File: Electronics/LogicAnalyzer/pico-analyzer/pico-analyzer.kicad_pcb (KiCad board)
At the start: 4 copper layers, 78.7 x 76.2 mm, 69 parts, among them J1 Channels 0-5, J2 Channels 6-11, J3 Channels 12-17, J4 Channels 18-23, J5 USB_C_Receptacle_USB2.0_16P, SW1 SW_DP3T, U1 TXU0104PW, U2 TXU0104PW, U3 TXU0104PW, U4 TXU0104PW, U5 TXU0104PW, U6 TXU0104PW, U7 RP2040_Stamp

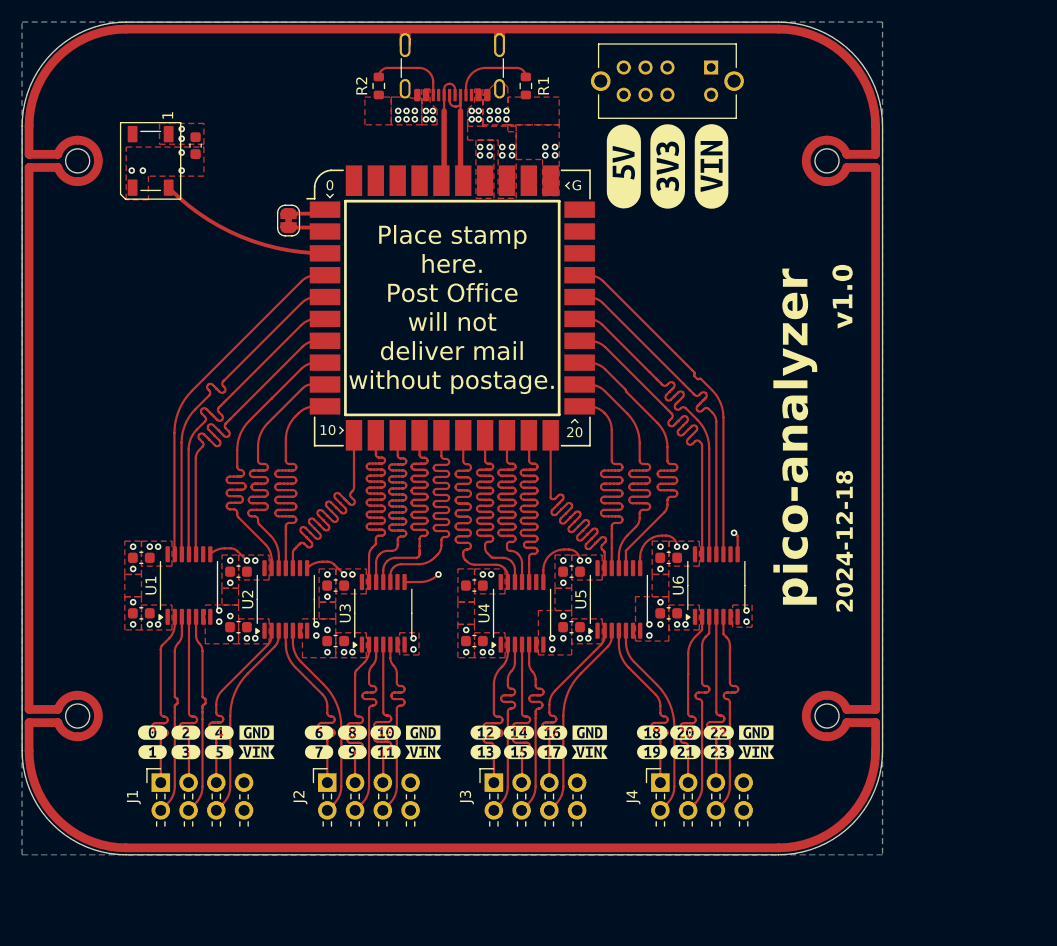
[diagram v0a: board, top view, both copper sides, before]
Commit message: Working on pico-analyzer v2
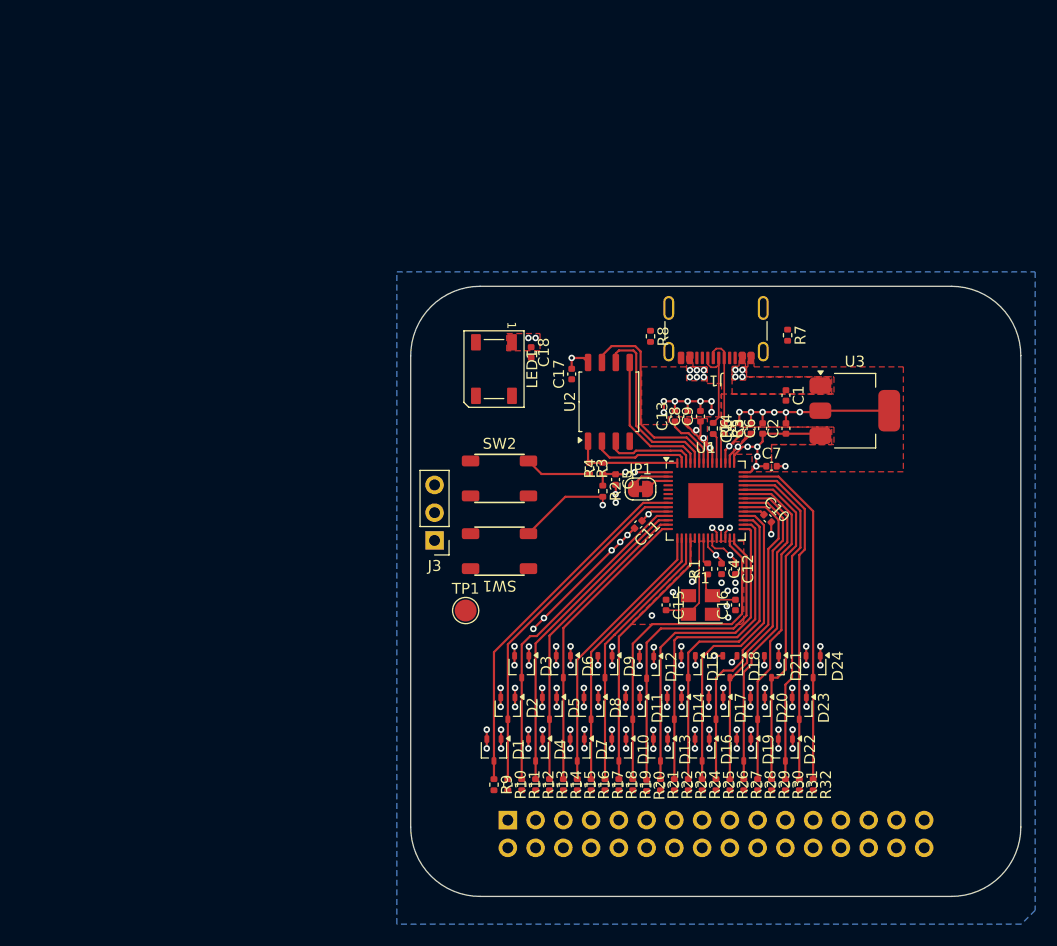
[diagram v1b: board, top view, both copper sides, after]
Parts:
- removed J4: Channels 18-23, pico-analyzer:PinHeader_2x04_P2.54mm_Horizontal
- removed J5: USB_C_Receptacle_USB2.0_16P, pico-analyzer:USB_C_Receptacle_GCT_USB4215-xx-A_16P
- removed MH (x4): MountingHole_2.2mm_M2_DIN965, MountingHole:MountingHole_2.2mm_M2_DIN965
- removed U4, U5, U6: TXU0104PW, Package_SO:TSSOP-14_4.4x5mm_P0.65mm
- removed U7: RP2040_Stamp, pico-analyzer:RP2xxx_Stamp_SMD
- removed kibuzzard-67631203: G***, kibuzzard-67631203
- removed kibuzzard-6763120A: G***, kibuzzard-6763120A
- removed kibuzzard-67631217: G***, kibuzzard-67631217
- removed kibuzzard-67631277: G***, kibuzzard-67631277
- removed kibuzzard-6763127F: G***, kibuzzard-6763127F
- removed kibuzzard-67631289: G***, kibuzzard-67631289
- removed kibuzzard-6763155B: G***, kibuzzard-6763155B
- removed kibuzzard-67631565: G***, kibuzzard-67631565
- removed kibuzzard-6763156D: G***, kibuzzard-6763156D
- removed kibuzzard-67631578: G***, kibuzzard-67631578
- removed kibuzzard-67631580: G***, kibuzzard-67631580
- removed kibuzzard-67631586: G***, kibuzzard-67631586
- removed kibuzzard-676315DE (x4): G***, kibuzzard-676315DE
- removed kibuzzard-67631617 (x4): G***, kibuzzard-67631617
- removed kibuzzard-67631703: G***, kibuzzard-67631703
- removed kibuzzard-6763170A: G***, kibuzzard-6763170A
- removed kibuzzard-67631748: G***, kibuzzard-67631748
- removed kibuzzard-6763175E: G***, kibuzzard-6763175E
- removed kibuzzard-67631765: G***, kibuzzard-67631765
- removed kibuzzard-67631771: G***, kibuzzard-67631771
- removed kibuzzard-676317E0: G***, kibuzzard-676317E0
- removed kibuzzard-676317E5: G***, kibuzzard-676317E5
- removed kibuzzard-676317E9: G***, kibuzzard-676317E9
- removed kibuzzard-676317ED: G***, kibuzzard-676317ED
- removed kibuzzard-676317F6: G***, kibuzzard-676317F6
- removed kibuzzard-67631801: G***, kibuzzard-67631801
- removed kibuzzard-67632017: G***, kibuzzard-67632017
- removed kibuzzard-6763201C: G***, kibuzzard-6763201C
- removed kibuzzard-67632021: G***, kibuzzard-67632021
- added C14: 0.1µF, Capacitor_SMD:C_0402_1005Metric, F.Cu at (141.8, 88.0)
- added C15: 15pF, Capacitor_SMD:C_0402_1005Metric, F.Cu at (135.1, 104.1)
- added C16: 15pF, Capacitor_SMD:C_0402_1005Metric, F.Cu at (141.5, 104.1)
- added C17: 0.1µF, Capacitor_SMD:C_0402_1005Metric, F.Cu at (126.5, 83.0)
- added C18: 0.1µF, Capacitor_SMD:C_0402_1005Metric, F.Cu at (122.8, 81.0)
- added D10: BAV99, Package_TO_SOT_SMD:SOT-323_SC-70, F.Cu at (130.8, 117.4)
- added D11: BAV99, Package_TO_SOT_SMD:SOT-323_SC-70, F.Cu at (132.1, 113.6)
- added D12: BAV99, Package_TO_SOT_SMD:SOT-323_SC-70, F.Cu at (133.3, 109.9)
- added D13: BAV99, Package_TO_SOT_SMD:SOT-323_SC-70, F.Cu at (134.6, 117.4)
- added D14: BAV99, Package_TO_SOT_SMD:SOT-323_SC-70, F.Cu at (135.9, 113.6)
- added D15: BAV99, Package_TO_SOT_SMD:SOT-323_SC-70, F.Cu at (137.2, 109.8)
- added D16: BAV99, Package_TO_SOT_SMD:SOT-323_SC-70, F.Cu at (138.4, 117.4)
- added D17: BAV99, Package_TO_SOT_SMD:SOT-323_SC-70, F.Cu at (139.7, 113.6)
- added D18: BAV99, Package_TO_SOT_SMD:SOT-323_SC-70, F.Cu at (141.0, 109.8)
- added D19: BAV99, Package_TO_SOT_SMD:SOT-323_SC-70, F.Cu at (142.2, 117.4)
- added D2: BAV99, Package_TO_SOT_SMD:SOT-323_SC-70, F.Cu at (120.7, 113.6)
- added D20: BAV99, Package_TO_SOT_SMD:SOT-323_SC-70, F.Cu at (143.5, 113.6)
- added D21: BAV99, Package_TO_SOT_SMD:SOT-323_SC-70, F.Cu at (144.8, 109.8)
- added D22: BAV99, Package_TO_SOT_SMD:SOT-323_SC-70, F.Cu at (146.1, 117.4)
- added D23: BAV99, Package_TO_SOT_SMD:SOT-323_SC-70, F.Cu at (147.3, 113.6)
- added D24: BAV99, Package_TO_SOT_SMD:SOT-323_SC-70, F.Cu at (148.6, 109.8)
- added D3: BAV99, Package_TO_SOT_SMD:SOT-323_SC-70, F.Cu at (121.9, 109.8)
- added D4: BAV99, Package_TO_SOT_SMD:SOT-323_SC-70, F.Cu at (123.2, 117.4)
- added D5: BAV99, Package_TO_SOT_SMD:SOT-323_SC-70, F.Cu at (124.5, 113.6)
- added D6: BAV99, Package_TO_SOT_SMD:SOT-323_SC-70, F.Cu at (125.7, 109.8)
- added D7: BAV99, Package_TO_SOT_SMD:SOT-323_SC-70, F.Cu at (127.0, 117.4)
- added D8: BAV99, Package_TO_SOT_SMD:SOT-323_SC-70, F.Cu at (128.3, 113.6)
- added D9: BAV99, Package_TO_SOT_SMD:SOT-323_SC-70, F.Cu at (129.5, 109.8)
- added LED1: WS2812B, LED_SMD:LED_WS2812B_PLCC4_5.0x5.0mm_P3.2mm, F.Cu at (119.4, 82.5)
- added R10: 220, Resistor_SMD:R_0402_1005Metric, F.Cu at (120.7, 120.6)
- added R11: 220, Resistor_SMD:R_0402_1005Metric, F.Cu at (121.9, 120.6)
- added R12: 220, Resistor_SMD:R_0402_1005Metric, F.Cu at (123.2, 120.6)
- added R13: 220, Resistor_SMD:R_0402_1005Metric, F.Cu at (124.5, 120.6)
- added R14: 220, Resistor_SMD:R_0402_1005Metric, F.Cu at (125.7, 120.6)
- added R15: 220, Resistor_SMD:R_0402_1005Metric, F.Cu at (127.0, 120.6)
- added R16: 220, Resistor_SMD:R_0402_1005Metric, F.Cu at (128.3, 120.6)
- added R17: 220, Resistor_SMD:R_0402_1005Metric, F.Cu at (129.5, 120.6)
- added R18: 220, Resistor_SMD:R_0402_1005Metric, F.Cu at (130.8, 120.6)
- added R19: 220, Resistor_SMD:R_0402_1005Metric, F.Cu at (132.1, 120.6)
- added R20: 220, Resistor_SMD:R_0402_1005Metric, F.Cu at (133.3, 120.7)
- added R21: 220, Resistor_SMD:R_0402_1005Metric, F.Cu at (134.6, 120.6)
- added R22: 220, Resistor_SMD:R_0402_1005Metric, F.Cu at (135.9, 120.6)
- added R23: 220, Resistor_SMD:R_0402_1005Metric, F.Cu at (137.2, 120.6)
- added R24: 220, Resistor_SMD:R_0402_1005Metric, F.Cu at (138.4, 120.6)
- added R25: 220, Resistor_SMD:R_0402_1005Metric, F.Cu at (139.7, 120.6)
- added R26: 220, Resistor_SMD:R_0402_1005Metric, F.Cu at (141.0, 120.6)
- added R27: 220, Resistor_SMD:R_0402_1005Metric, F.Cu at (142.2, 120.6)
- added R28: 220, Resistor_SMD:R_0402_1005Metric, F.Cu at (143.5, 120.6)
- added R29: 220, Resistor_SMD:R_0402_1005Metric, F.Cu at (144.8, 120.6)
- added R3: 1K, Resistor_SMD:R_0402_1005Metric, F.Cu at (128.1, 91.6)
- added R30: 220, Resistor_SMD:R_0402_1005Metric, F.Cu at (146.1, 120.6)
- added R31: 220, Resistor_SMD:R_0402_1005Metric, F.Cu at (147.3, 120.6)
- added R32: 220, Resistor_SMD:R_0402_1005Metric, F.Cu at (148.6, 120.6)
- added R4: 10K, Resistor_SMD:R_0402_1005Metric, F.Cu at (129.3, 91.6)
- added R5: 27R, Resistor_SMD:R_0402_1005Metric, F.Cu at (140.5, 88.0)
- added R6: 27R, Resistor_SMD:R_0402_1005Metric, F.Cu at (139.4, 88.0)
- added R7: 5K1, Resistor_SMD:R_0402_1005Metric, F.Cu at (146.3, 79.5)
- added R8: 5K1, Resistor_SMD:R_0402_1005Metric, F.Cu at (133.7, 79.6)
- added R9: 220, Resistor_SMD:R_0402_1005Metric, F.Cu at (119.4, 120.6)
- added SW2: BOOT, UPL-Switches:Button_Push_SPST_C&K_PTS647Sx38SMTR2LFS, F.Cu at (119.9, 92.6)
- added TP1: TESTEN, TestPoint:TestPoint_Pad_D2.0mm, F.Cu at (116.8, 104.6)
- added Y1: ABM8-272-T3, Crystal:Crystal_SMD_Abracon_ABM8G-4Pin_3.2x2.5mm, F.Cu at (138.3, 104.1)
- C1: value 100nF -> 4.7µF; footprint Capacitor_SMD:C_0603_1608Metric -> Capacitor_SMD:C_0402_1005Metric
- C10, C11, C13, C4, C5, C6, C7, C8, C9: value C_Small -> 0.1µF; footprint Capacitor_SMD:C_0603_1608Metric -> Capacitor_SMD:C_0402_1005Metric
- C12, C3: value C_Small -> 1µF; footprint Capacitor_SMD:C_0603_1608Metric -> Capacitor_SMD:C_0402_1005Metric
- C2: value C_Small -> 4.7µF; footprint Capacitor_SMD:C_0603_1608Metric -> Capacitor_SMD:C_0402_1005Metric
- D1: value WS2812B -> BAV99; footprint LED_SMD:LED_WS2812B_PLCC4_5.0x5.0mm_P3.2mm -> Package_TO_SOT_SMD:SOT-323_SC-70
- J1: value Channels 0-5 -> USB_C_Receptacle_USB2.0_16P; footprint pico-analyzer:PinHeader_2x04_P2.54mm_Horizontal -> pico-analyzer:USB_C_Receptacle_GCT_USB4215-xx-A_16P
- J2: value Channels 6-11 -> Conn_02x16_Odd_Even; footprint pico-analyzer:PinHeader_2x04_P2.54mm_Horizontal -> Connector_PinHeader_2.54mm:PinHeader_2x16_P2.54mm_Horizontal; moved to B.Cu
- J3: value Channels 12-17 -> DEBUG; footprint pico-analyzer:PinHeader_2x04_P2.54mm_Horizontal -> Connector_PinHeader_2.54mm:PinHeader_1x03_P2.54mm_Vertical
- R1: value 5K1 -> 1K; footprint Resistor_SMD:R_0603_1608Metric -> Resistor_SMD:R_0402_1005Metric
- R2: value 5K1 -> 10K; footprint Resistor_SMD:R_0603_1608Metric -> Resistor_SMD:R_0402_1005Metric
- SW1: value SW_DP3T -> RESET; footprint pico-analyzer:EG2315A -> UPL-Switches:Button_Push_SPST_C&K_PTS647Sx38SMTR2LFS
- U1: value TXU0104PW -> RP2040; footprint Package_SO:TSSOP-14_4.4x5mm_P0.65mm -> Package_DFN_QFN:QFN-56-1EP_7x7mm_P0.4mm_EP3.2x3.2mm
- U2: value TXU0104PW -> W25Q128JVS; footprint Package_SO:TSSOP-14_4.4x5mm_P0.65mm -> Package_SO:SOIC-8_5.23x5.23mm_P1.27mm
- U3: value TXU0104PW -> AP2114HA-3.3TRG1; footprint Package_SO:TSSOP-14_4.4x5mm_P0.65mm -> Package_TO_SOT_SMD:SOT-223-3_TabPin2
- moved J1 66.1 mm to (139.7, 78.1), turned to 180 degrees
- moved D1 62.4 mm to (119.4, 117.4)
- moved C2 60.2 mm to (146.1, 88.0), turned to 90 degrees
- moved C1 58.7 mm to (146.1, 85.0)
- moved C3 58.3 mm to (142.9, 88.0), turned to 90 degrees
- moved SW1 48.3 mm to (119.9, 99.2)
- moved U1 47.9 mm to (138.8, 94.6), turned to 0 degrees
- moved R1 47.2 mm to (138.9, 100.8), turned to 90 degrees
- moved U3 47.0 mm to (152.4, 86.4), turned to 0 degrees
- moved C4 44.2 mm to (140.2, 100.8), turned to -90 degrees
- moved C7 43.0 mm to (144.8, 91.4), turned to 0 degrees
- moved R2 42.4 mm to (129.3, 93.7)
- moved C6 41.6 mm to (144.0, 88.0), turned to 90 degrees
- moved JP1 40.5 mm to (132.8, 93.5), turned to 0 degrees
- moved C5 37.1 mm to (130.5, 92.7), turned to -90 degrees
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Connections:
- C1 pad 1: +5V -> VBUS
- C11 pad 1: V_{ref} -> +3V3
- C12 pad 1: +3V3 -> +1V1
- C13 pad 1: V_{ref} -> +1V1
- C3 pad 1: V_{ref} -> +3V3
- C5 pad 1: V_{ref} -> +3V3
- C7 pad 1: V_{ref} -> +3V3
- C9 pad 1: V_{ref} -> +3V3
- D1 pad 1: +5V -> GND
- D1 pad 2: unconnected-(D1-DOUT-Pad2) -> +3V3
- D1 pad 3: GND -> /Level Translation/I0
- J2 pad 1: /Level Translation/C6 -> /Level Translation/C1
- J2 pad 2: /Level Translation/C7 -> /Level Translation/C0
- J2 pad 3: /Level Translation/C8 -> /Level Translation/C3
- J2 pad 4: /Level Translation/C9 -> /Level Translation/C2
- J2 pad 5: /Level Translation/C10 -> /Level Translation/C5
- J2 pad 6: /Level Translation/C11 -> /Level Translation/C4
- J2 pad 7: GND -> /Level Translation/C7
- J2 pad 8: V_{in} -> /Level Translation/C6
- J3 pad 1: /Level Translation/C12 -> Net-(J3-Pin_1)
- J3 pad 2: /Level Translation/C13 -> Net-(J3-Pin_2)
- J3 pad 3: /Level Translation/C14 -> GND
- JP1 pad 2: Net-(JP1-B) -> /EXT_IN
- R1 pad 2: GND -> Net-(U1-XOUT)
- R2 pad 1: Net-(J5-CC2) -> +3V3
- R2 pad 2: GND -> Net-(U1-RUN)
- SW1 pad 1: V_{in} -> GND
- SW1 pad 2: V_{ref} -> Net-(U1-RUN)
- U1 pad 1: V_{ref} -> +3V3
- U1 pad 10: /Level Translation/I3 -> +3V3
- U1 pad 12: /Level Translation/I1 -> /Level Translation/I3
- U1 pad 13: /Level Translation/I0 -> /Level Translation/I4
- U1 pad 14: +3V3 -> /Level Translation/I5
- U1 pad 2: /Level Translation/C0 -> Net-(JP1-A)
- U1 pad 3: /Level Translation/C1 -> /EXT_IN
- U1 pad 4: /Level Translation/C2 -> unconnected-(U1-GPIO2-Pad4)
- U1 pad 5: /Level Translation/C3 -> unconnected-(U1-GPIO3-Pad5)
- U1 pad 7: GND -> Net-(LED1-DIN)
- U1 pad 8: +3V3 -> /Level Translation/I0
- U1 pad 9: unconnected-(U1-NC-Pad9) -> /Level Translation/I1
- U2 pad 1: V_{ref} -> /~{QSPI_CS}
- U2 pad 2: /Level Translation/C4 -> /QSIP_SD1
- U2 pad 3: /Level Translation/C5 -> /QSIP_SD2
- U2 pad 4: /Level Translation/C6 -> GND
- U2 pad 5: /Level Translation/C7 -> /QSIP_SD0
- U2 pad 6: unconnected-(U2-NC-Pad6) -> /QSIP_SCLK
- U2 pad 7: GND -> /QSIP_SD3
- U3 pad 1: V_{ref} -> VBUS
- U3 pad 2: /Level Translation/C8 -> GND
- U3 pad 3: /Level Translation/C9 -> +3V3
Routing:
- net GND: track 2.68 -> 83.1 mm, vias 54 -> 77
- net +3V3: track 30.4 -> 84.1 mm, vias 18 -> 58
- net Net-(J3-Pin_2): track 0.00 -> 31.7 mm, vias 0 -> 1
- net Net-(J3-Pin_1): track 0.00 -> 31.6 mm, vias 0 -> 1
- net Net-(U1-RUN): track 0.00 -> 23.0 mm, vias 0 -> 2
- net /Level Translation/C23: track 20.2 -> 0.00 mm
- net /Level Translation/C21: track 20.1 -> 0.00 mm
- net /Level Translation/C20: track 19.8 -> 0.00 mm
- net /QSIP_SD3: track 0.00 -> 18.9 mm
- net /Level Translation/C2: track 18.7 -> 0.00 mm
- net /Level Translation/C22: track 18.7 -> 0.00 mm
- net /Level Translation/C14: track 18.7 -> 0.00 mm
- net /Level Translation/C10: track 18.7 -> 0.00 mm
- net /Level Translation/C0: track 18.6 -> 0.00 mm
- net /Level Translation/C3: track 18.6 -> 0.00 mm
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- added copper zone on In2.Cu, net +1V1
- added copper zone on F.Cu, net VBUS
- added copper zone on In2.Cu, net VBUS
- removed copper zone on F.Cu, net +5V
- removed copper zone on In2.Cu, net +5V
- removed copper zone on In2.Cu, net V_{in}
- removed copper zone on F.Cu, net V_{ref}
- removed copper zone on In2.Cu, net V_{ref}
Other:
- board size 78.7 x 76.2 mm -> 55.8 x 55.8 mm
- board text removed: "2024-12-18"
- board text removed: "Place stamp here. Post Office will not deliver mail without postage."
- board text removed: "pico-analyzer"
- board text removed: "v1.0"
